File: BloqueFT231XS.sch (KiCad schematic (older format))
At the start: 11 parts, among them U3 FT231XS

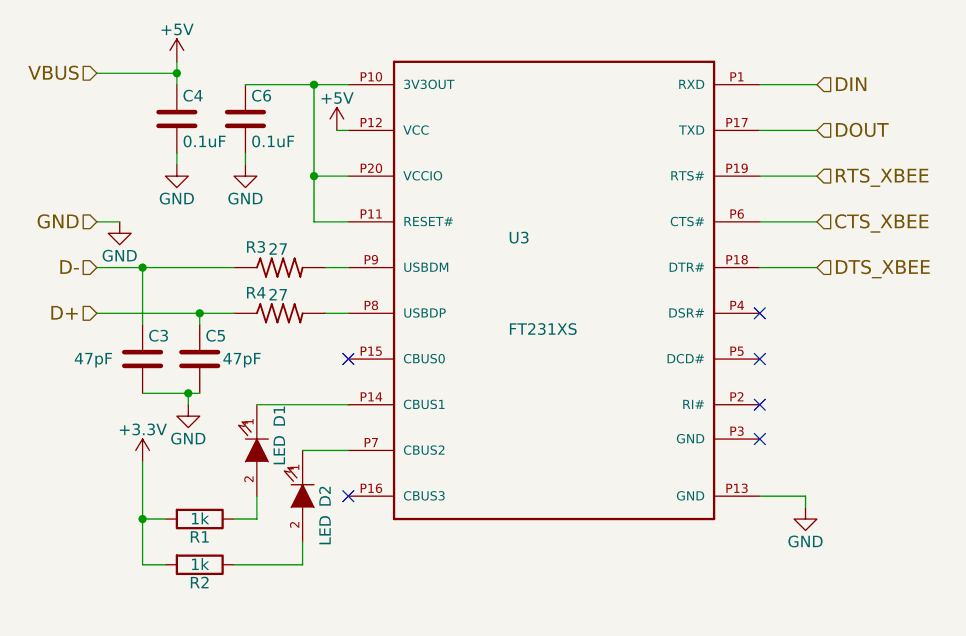
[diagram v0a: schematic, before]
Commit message: QuitandoBloques
Se le quitan las hojas de bloques
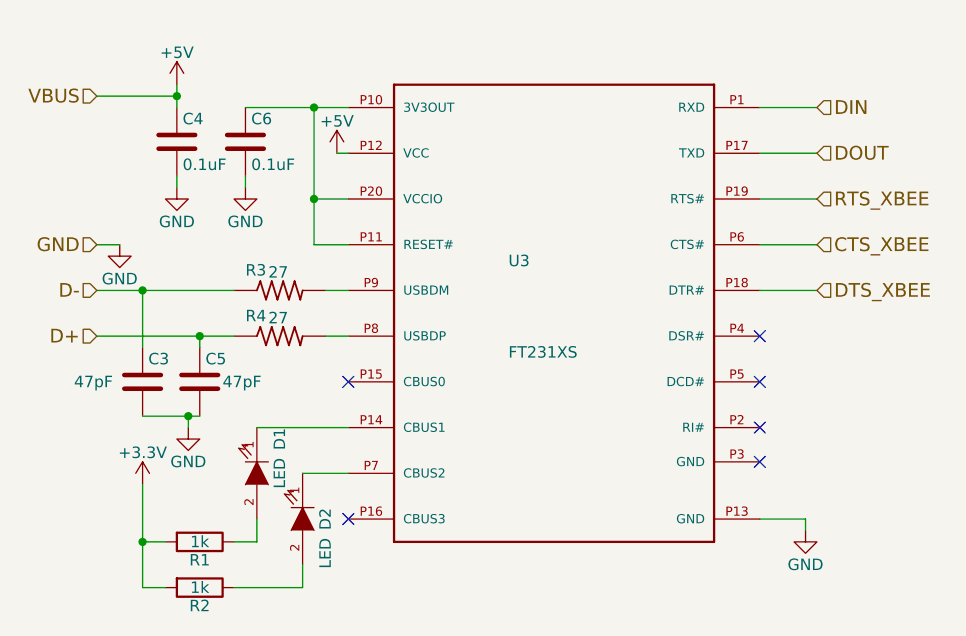
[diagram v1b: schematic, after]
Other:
- moved on the sheet: C3, C4, C5, C6, D1, D2, R1, R2, R3, R4, U3
